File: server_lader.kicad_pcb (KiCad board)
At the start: 2 copper layers, 100 x 160 mm, 76 parts, among them IC1 ATMEGA168PA-A, IC2 DAC8560, P1 5V_Vbatt, P10 DISPLAY_STECKER, P11 on/off, P12 A_regulation_out, P2 DISPLAY_STECKER, P3 CONN_02X03, P4 I2C, P5 IP+, P6 IP-, P7 UART, P8 CONN_01X01, P9 Drehrad, U1 ACS758, U2 LTV-356T, U3 ADUM3441, U4 RD-0512D, U5 TPS7A4901, U6 OPA188, U7 LM4040, Y1 RESONATEUR

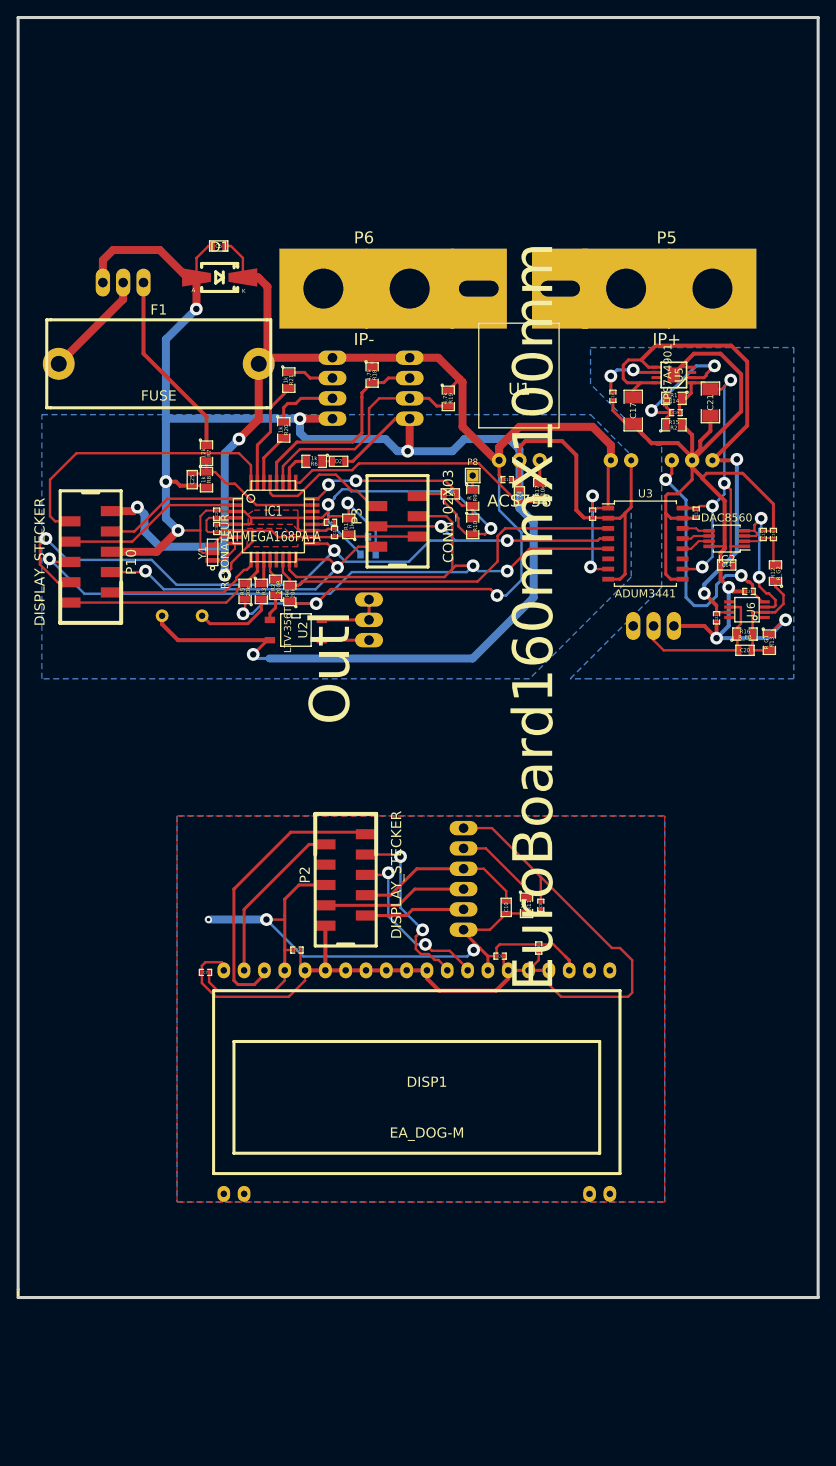
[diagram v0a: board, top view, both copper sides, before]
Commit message: für Fertigung vorbereitet
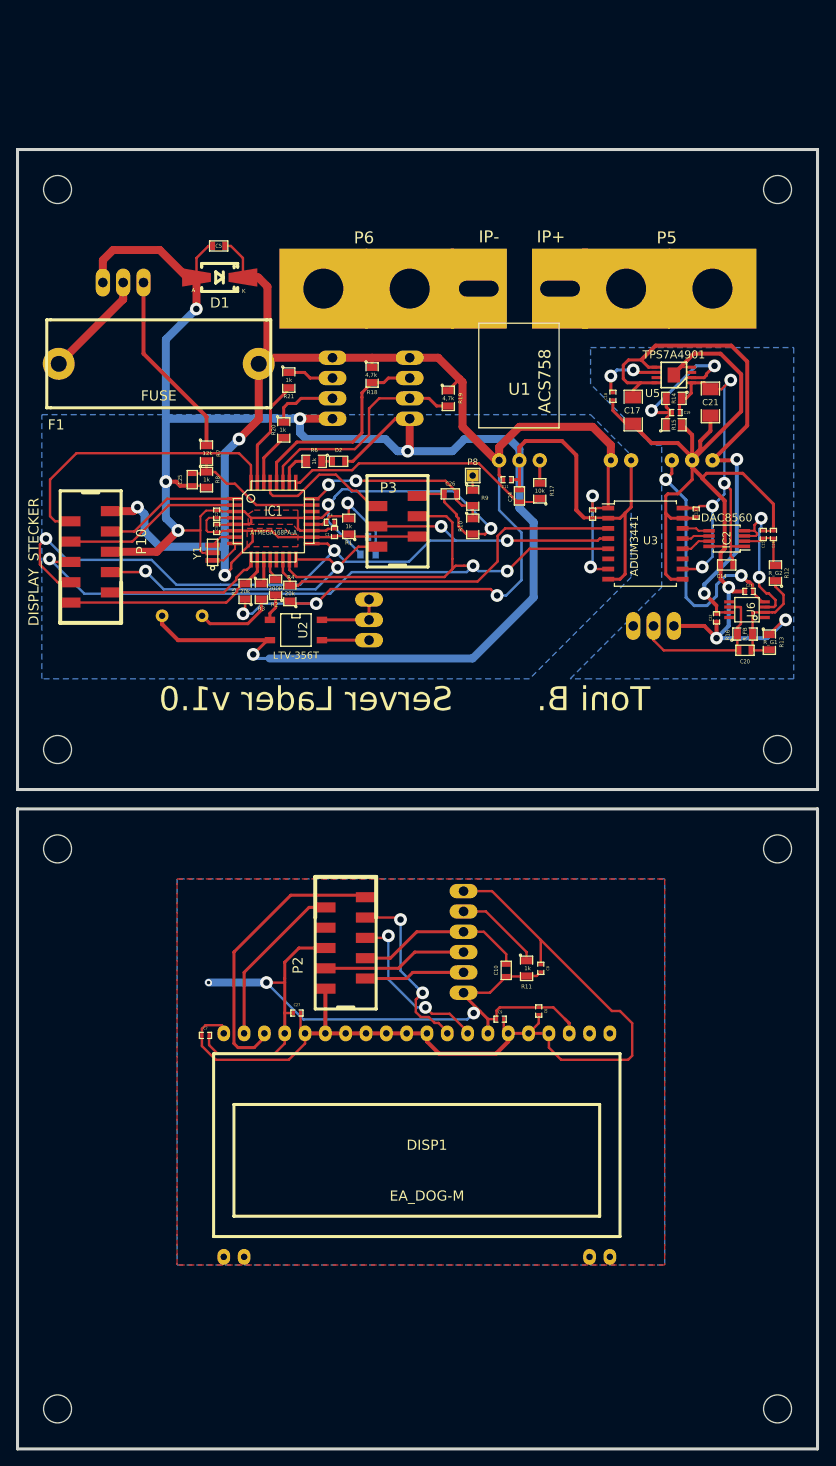
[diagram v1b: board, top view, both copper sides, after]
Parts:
- removed the Outl at (162.6, 173.4)
- added Outl: EuroBoard_halb_Type-I_100mmX80mm_holes, EuroBoard_Outline:EuroBoard_halb_Type-I_100mmX80mm_holes, F.Cu at (62.5, 192.3)
- added Outl: EuroBoard_halb_Type-I_100mmX80mm_holes, EuroBoard_Outline:EuroBoard_halb_Type-I_100mmX80mm_holes, F.Cu at (62.5, 109.9)
- moved C10 7.87 mm to (123.6, 132.5)
- moved C27 7.87 mm to (97.4, 137.8)
- moved C6 7.87 mm to (127.6, 137.5)
- moved C7 7.87 mm to (86.0, 140.6)
- moved C8 7.87 mm to (127.9, 132.2)
- moved C9 7.87 mm to (122.8, 138.6)
- moved DISP1 7.87 mm to (113.7, 155.6)
- moved P2 7.87 mm to (103.5, 128.4)
- moved P9 7.87 mm to (118.2, 128.9)
- moved R11 7.87 mm to (126.1, 132.2)
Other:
- board size 100 x 160 mm -> 100 x 80 mm
- board text added: "Toni B. Server Lader v1.0"
